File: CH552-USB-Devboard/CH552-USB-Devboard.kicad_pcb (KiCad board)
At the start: 2 copper layers, 22 x 40.5 mm, 26 parts, among them J1 Conn_01x11_Male, J2 Conn_01x11_Male, J3 USB_C_Receptacle, Q1 CPH6337, SW1 SW_Push, SW2 SW_Push, U1 CH552T, U2 CH552G, U3 MIC5504-3.3YM5, Y1 Crystal

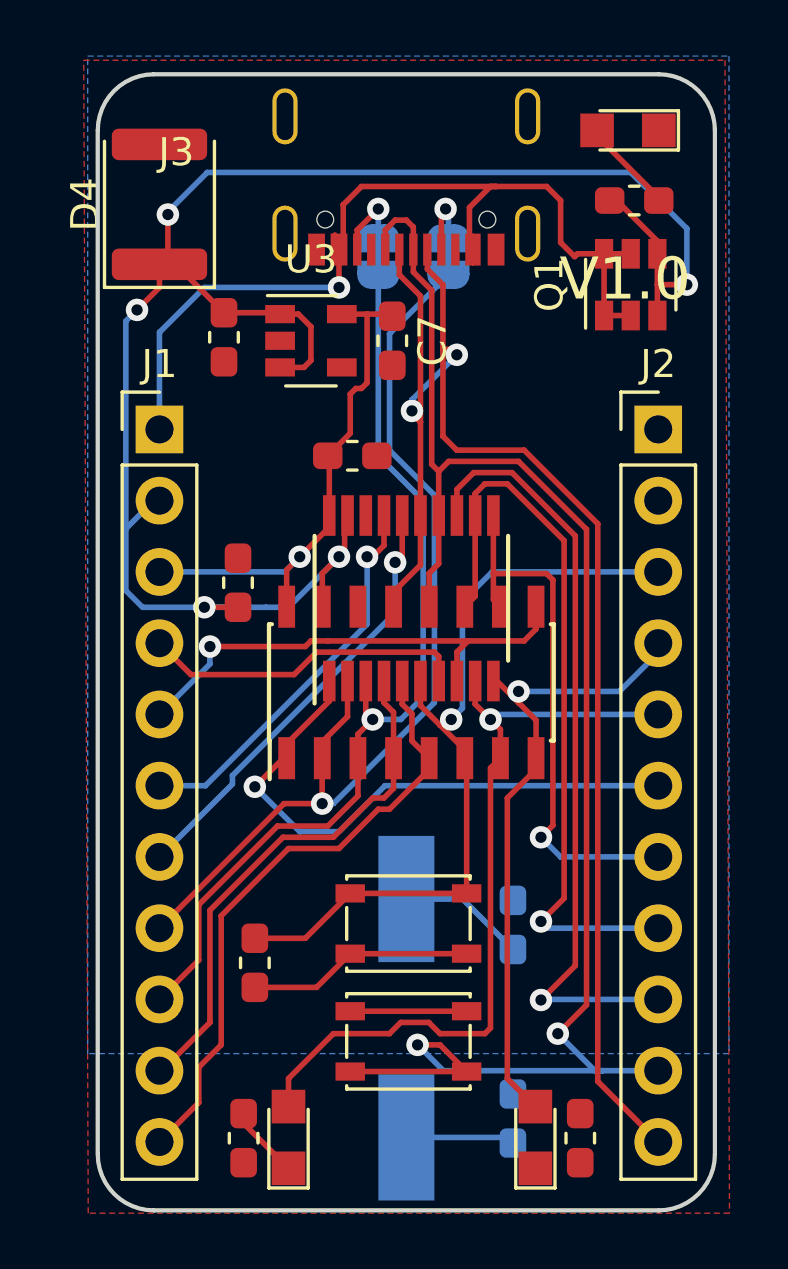
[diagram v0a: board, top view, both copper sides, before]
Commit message: update and created test grebers
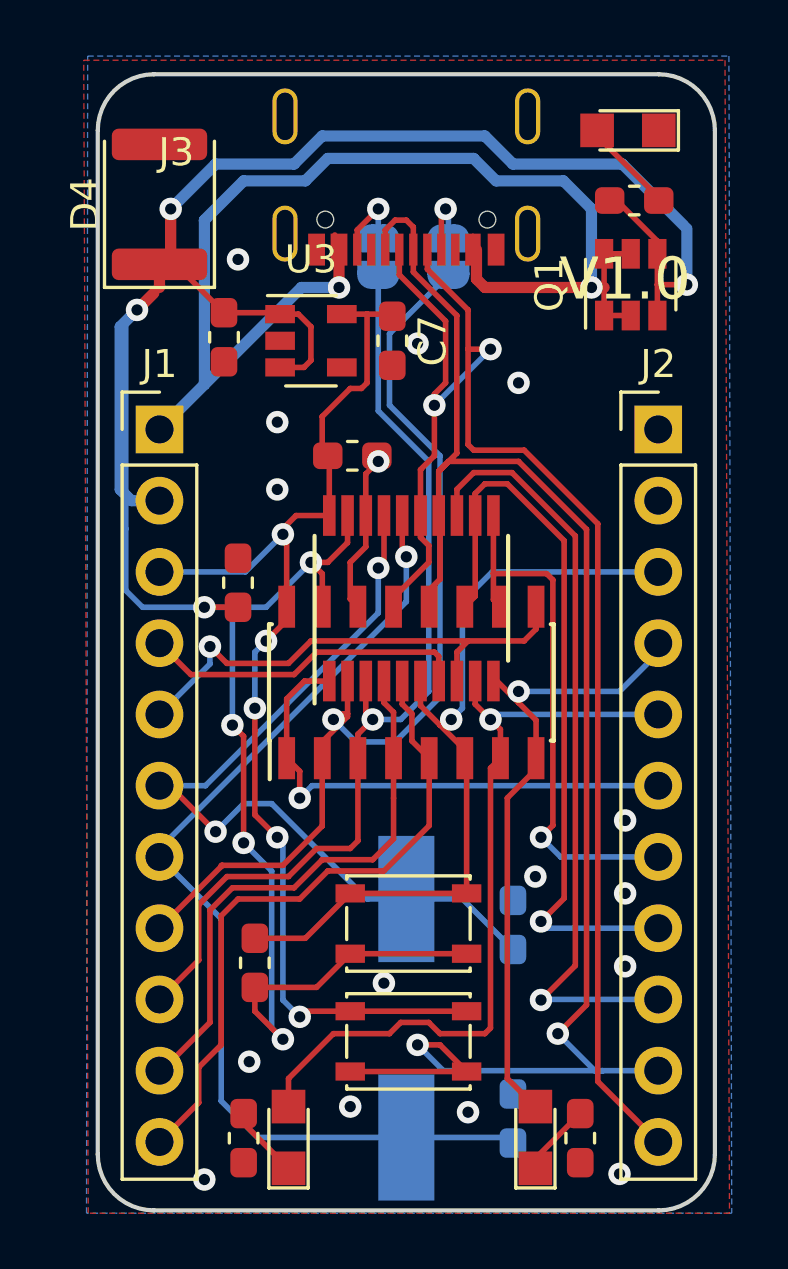
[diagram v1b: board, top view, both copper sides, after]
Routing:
- net VCC: track 74.0 -> 104.3 mm, vias 5 -> 8
- net +3V3: track 23.0 -> 41.5 mm, vias 1 -> 5
- net /P1.3: track 19.6 -> 36.5 mm
- net VBUS: track 32.7 -> 46.0 mm, vias 1 -> 2
- net /P1.2: track 18.6 -> 30.6 mm, vias 1 -> 2
- net GND: track 0.00 -> 5.71 mm, vias 0 -> 16
- net Net-(D1-Pad1): track 0.00 -> 2.61 mm
- net /P3.2: track 20.7 -> 18.5 mm
- net /P1.7: track 22.1 -> 23.3 mm
- net /P1.5: track 33.5 -> 34.6 mm
- net /P1.6: track 18.8 -> 19.9 mm
- net /P3.6: track 58.2 -> 58.8 mm
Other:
- net class power added: clearance 0.2, trace_width 0.4, via_dia 0.8, via_drill 0.4

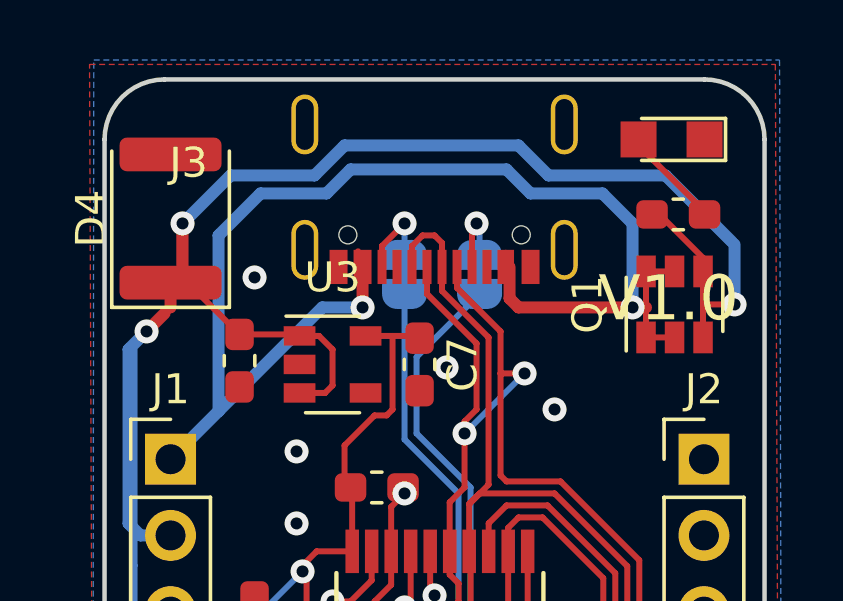
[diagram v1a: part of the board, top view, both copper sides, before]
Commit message: work on v2 silk
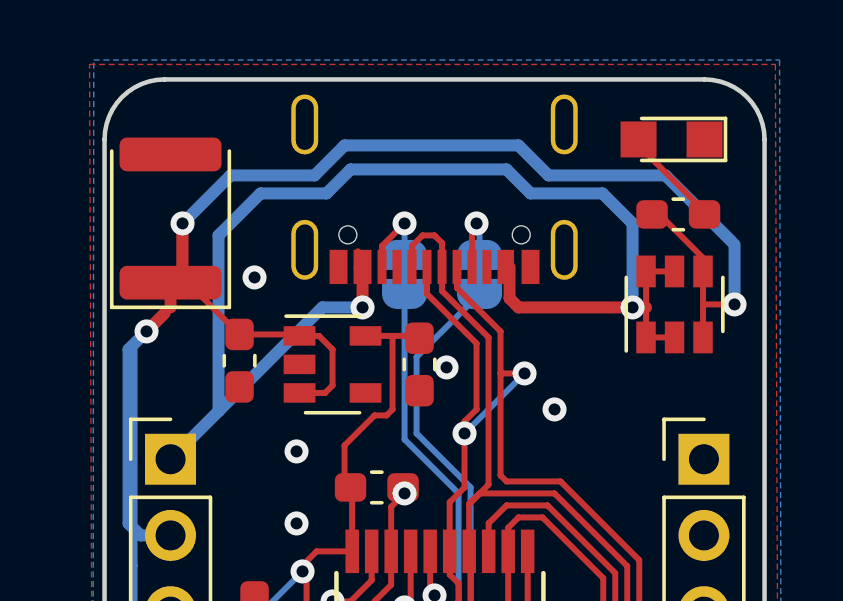
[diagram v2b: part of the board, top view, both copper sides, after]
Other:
- board text removed: "V1.0"
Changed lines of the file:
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@@
   (general
     (thickness 1.6)
-    (drawings 9)
+    (drawings 8)
     (tracks 425)
     (zones 0)
@@
     (34 B.Paste user hide)
     (35 F.Paste user hide)
-    (36 B.SilkS user hide)
-    (37 F.SilkS user hide)
-    (38 B.Mask user)
+    (36 B.SilkS user)
+    (37 F.SilkS user)
+    (38 B.Mask user hide)
     (39 F.Mask user hide)
     (40 Dwgs.User user)
@@
     (46 B.CrtYd user)
     (47 F.CrtYd user)
-    (48 B.Fab user hide)
-    (49 F.Fab user hide)
+    (48 B.Fab user)
+    (49 F.Fab user)
   )
   (setup
@@
     (pad_to_mask_clearance 0.2)
     (aux_axis_origin 0 0)
-    (visible_elements 7FE8FF1F)
+    (visible_elements 7FFEFFFF)
     (pcbplotparams
       (layerselection 0x010fc_ffffffff)
@@
       (drillshape 0)
       (scaleselection 1)
-      (outputdirectory "CHUSBIE552v2_0/"))
+      (outputdirectory "ArtandSilks/"))
   )
   (net 0 "")
@@
     (tags SOT-23-5)
     (attr smd)
-    (fp_text reference U3 (at 0 -2.9) (layer F.SilkS)
+    (fp_text reference U3 (at 0 -2.9) (layer F.SilkS) hide
       (effects (font (size 1 1) (thickness 0.15)))
     )
@@
     (tags "capacitor handsolder")
     (attr smd)
-    (fp_text reference C7 (at 0 -1.43 270) (layer F.SilkS)
+    (fp_text reference C7 (at 0 -1.43 270) (layer F.SilkS) hide
       (effects (font (size 1 1) (thickness 0.15)))
     )
@@
     (descr "Through hole straight pin header, 1x11, 2.54mm pitch, single row")
     (tags "Through hole pin header THT 1x11 2.54mm single row")
-    (fp_text reference J1 (at 0 -2.33) (layer F.SilkS)
-      (effects (font (size 1 1) (thickness 0.15)))
-    )
-    (fp_text value Conn_01x11_Male (at 0 27.73) (layer F.Fab)
+    (fp_text reference J1 (at 0 -2.33) (layer F.SilkS) hide
+      (effects (font (size 1 1) (thickness 0.15)))
+    )
+    (fp_text value Conn_01x11_Male (at 0 27.73) (layer F.Fab) hide
       (effects (font (size 1 1) (thickness 0.15)))
     )
@@
     (descr "Through hole straight pin header, 1x11, 2.54mm pitch, single row")
     (tags "Through hole pin header THT 1x11 2.54mm single row")
-    (fp_text reference J2 (at 0 -2.33) (layer F.SilkS)
+    (fp_text reference J2 (at 0 -2.33) (layer F.SilkS) hide
       (effects (font (size 1 1) (thickness 0.15)))
     )
@@
     (tags diode)
     (attr smd)
-    (fp_text reference D4 (at 0 -2.65 90) (layer F.SilkS)
+    (fp_text reference D4 (at 0 -2.65 90) (layer F.SilkS) hide
       (effects (font (size 1 1) (thickness 0.15)))
     )
@@
     (tags "solder jumper open")
     (attr virtual)
-    (fp_text reference JP1 (at 0 1.8 270) (layer B.SilkS)
+    (fp_text reference JP1 (at 0 1.8 270) (layer B.SilkS) hide
       (effects (font (size 1 1) (thickness 0.15)) (justify mirror))
     )
@@
     (tags "solder jumper open")
     (attr virtual)
-    (fp_text reference JP2 (at 0 1.8 270) (layer B.SilkS)
+    (fp_text reference JP2 (at 0 1.8 270) (layer B.SilkS) hide
       (effects (font (size 1 1) (thickness 0.15)) (justify mirror))
     )
@@
     (tags SOT-23-6)
     (attr smd)
-    (fp_text reference Q1 (at 0 -2.9 90) (layer F.SilkS)
+    (fp_text reference Q1 (at 0 -2.9 90) (layer F.SilkS) hide
       (effects (font (size 1 1) (thickness 0.15)))
     )
@@
   (module footprint:VACON_CSP_USC16_TR (layer F.Cu)
     (at 85 66.68 180)
-    (fp_text reference J3 (at 8.2 2.9 180) (layer F.SilkS)
+    (fp_text reference J3 (at 8.2 2.9 180) (layer F.SilkS) hide
       (effects (font (size 1 1) (thickness 0.15)))
     )
@@
       (effects (font (size 1 1) (thickness 0.15)))
     )
-    (fp_text value SW_Push (at 0 2.6) (layer F.Fab)
+    (fp_text value SW_Push (at 0 2.6) (layer F.Fab) hide
       (effects (font (size 1 1) (thickness 0.15)))
     )
@@
       (effects (font (size 1 1) (thickness 0.15)))
     )
-    (fp_text value CH552G (at -4.51998 -0.038392 180) (layer F.Fab)
+    (fp_text value CH552G (at -4.51998 -0.038392 180) (layer F.Fab) hide
       (effects (font (size 1 1) (thickness 0.15)))
     )
@@
       (effects (font (size 1 1) (thickness 0.15)))
     )
-    (fp_text value CH552T (at 4.68002 1.220808 180) (layer F.Fab)
+    (fp_text value CH552T (at 4.68002 1.220808 180) (layer F.Fab) hide
       (effects (font (size 1 1) (thickness 0.15)))
     )
@@
   (gr_arc (start 94 99.5) (end 94 101.5) (angle -90) (layer Edge.Cuts) (width 0.15))
   (gr_arc (start 94 63) (end 96 63) (angle -90) (layer Edge.Cuts) (width 0.15))
-  (gr_text V1.0 (at 92.8 68.3) (layer F.SilkS)
-    (effects (font (size 1.5 1.5) (thickness 0.3)))
-  )
   (gr_line (start 94 101.5) (end 76 101.5) (layer Edge.Cuts) (width 0.15))
   (gr_line (start 96 63) (end 96 99.5) (layer Edge.Cuts) (width 0.15))
